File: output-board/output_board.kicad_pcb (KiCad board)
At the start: 2 copper layers, 35 parts, among them J1 Conn_Input, J2 3V3, J3 5V, J4 Channel 1-2, J5 Channel 5-6, J6 Channel 3-4, J7 Channel 7-8, U1 PCM1681

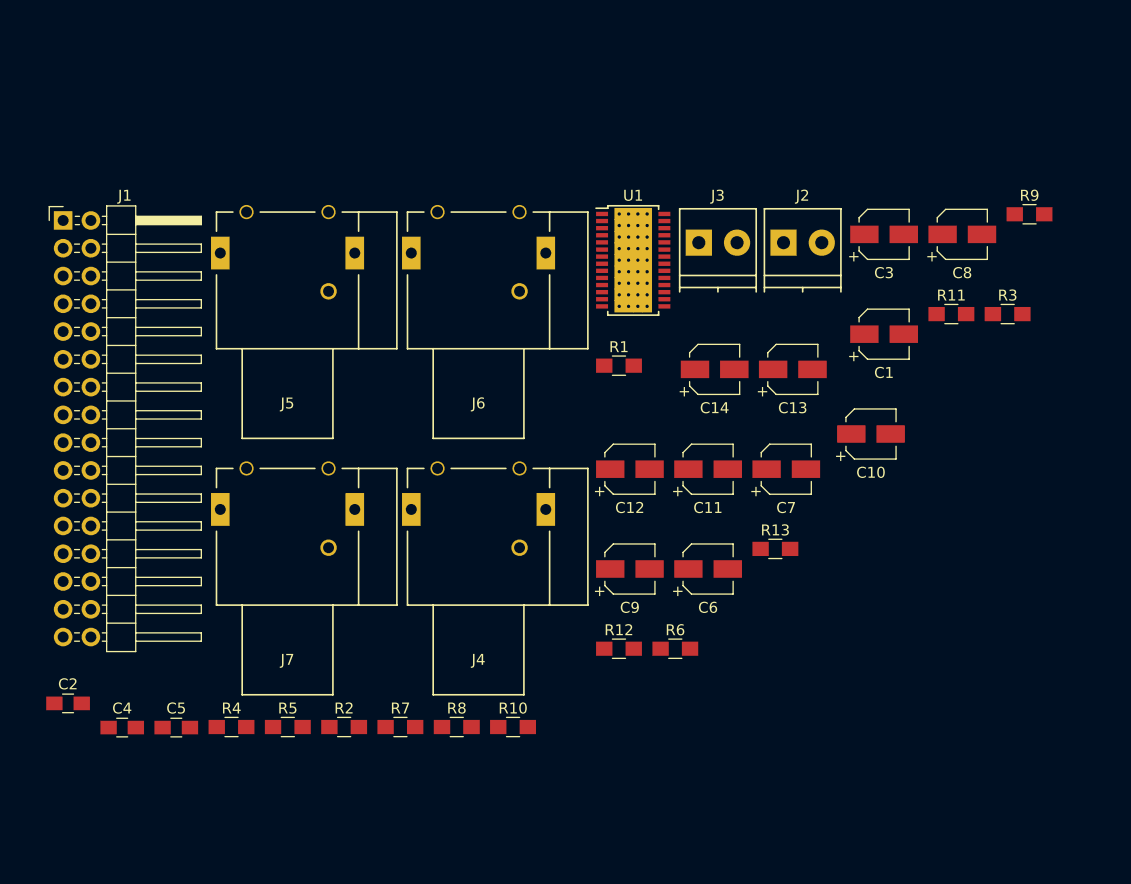
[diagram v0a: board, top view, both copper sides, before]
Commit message: update output-board
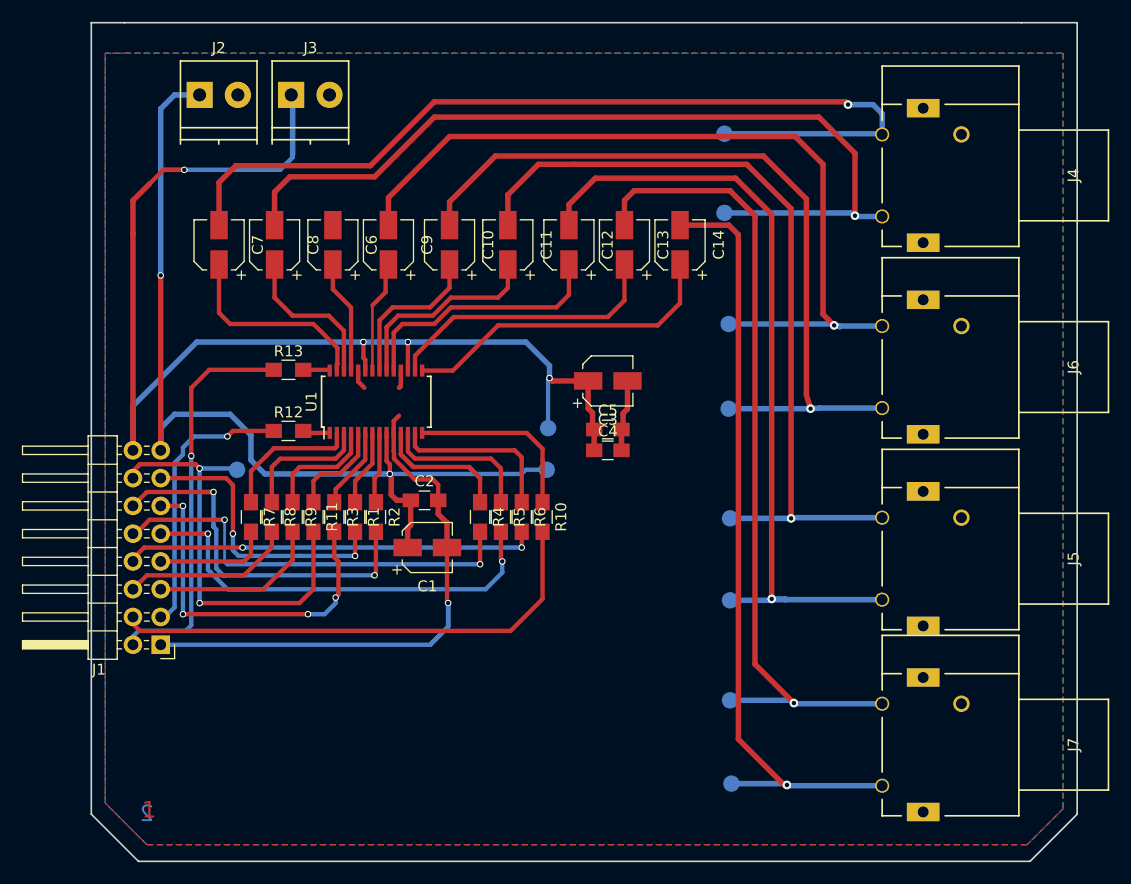
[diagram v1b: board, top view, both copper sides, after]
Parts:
- added TP1: Test_Point, Measurement_Points:Measurement_Point_Round-SMD-Pad_Small, B.Cu at (127.6, 91.9)
- added TP10: Test_Point, Measurement_Points:Measurement_Point_Round-SMD-Pad_Small, B.Cu at (172.7, 103.9)
- added TP11: Test_Point, Measurement_Points:Measurement_Point_Round-SMD-Pad_Small, B.Cu at (172.8, 120.7)
- added TP2: Test_Point, Measurement_Points:Measurement_Point_Round-SMD-Pad_Small, B.Cu at (156.0, 91.9)
- added TP3: Test_Point, Measurement_Points:Measurement_Point_Round-SMD-Pad_Small, B.Cu at (156.1, 88.1)
- added TP4: Test_Point, Measurement_Points:Measurement_Point_Round-SMD-Pad_Small, B.Cu at (172.2, 61.2)
- added TP5: Test_Point, Measurement_Points:Measurement_Point_Round-SMD-Pad_Small, B.Cu at (172.6, 78.6)
- added TP6: Test_Point, Measurement_Points:Measurement_Point_Round-SMD-Pad_Small, B.Cu at (172.2, 68.5)
- added TP7: Test_Point, Measurement_Points:Measurement_Point_Round-SMD-Pad_Small, B.Cu at (172.6, 86.4)
- added TP8: Test_Point, Measurement_Points:Measurement_Point_Round-SMD-Pad_Small, B.Cu at (172.7, 96.4)
- added TP9: Test_Point, Measurement_Points:Measurement_Point_Round-SMD-Pad_Small, B.Cu at (172.7, 113.0)
- J1: footprint Pin_Headers:Pin_Header_Angled_2x16_Pitch2.54mm -> Pin_Headers:Pin_Header_Angled_2x08_Pitch2.54mm
- moved R9 72.9 mm to (132.7, 96.3), turned to 270 degrees
- moved J5 69.6 mm to (199.1, 100.1), turned to 90 degrees
- moved J7 68.1 mm to (199.1, 117.1), turned to 90 degrees
- moved R3 64.3 mm to (136.5, 96.3), turned to 270 degrees
- moved J4 63.1 mm to (199.1, 65.0), turned to 90 degrees
- moved C8 62.9 mm to (131.1, 71.4), turned to 90 degrees
- moved R11 61.2 mm to (134.6, 96.3), turned to 270 degrees
- moved C7 55.8 mm to (126.0, 71.4), turned to 90 degrees
- moved J2 55.1 mm to (124.2, 57.7)
- moved C4 51.1 mm to (161.5, 90.2)
- moved J6 49.4 mm to (199.1, 82.5), turned to 90 degrees
- moved C5 48.0 mm to (161.5, 88.3)
- moved R13 47.4 mm to (132.3, 82.8)
- moved C1 46.1 mm to (145.0, 99.1)
- moved C6 45.4 mm to (136.4, 71.4), turned to 90 degrees
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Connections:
- C10 pad 1: /VOUT4 -> Net-(C10-Pad1)
- C10 pad 2: Net-(C10-Pad2) -> /VOUT4
- C11 pad 1: /VOUT5 -> Net-(C11-Pad1)
- C11 pad 2: Net-(C11-Pad2) -> /VOUT5
- C12 pad 1: /VOUT6 -> Net-(C12-Pad1)
- C12 pad 2: Net-(C12-Pad2) -> /VOUT6
- C13 pad 1: /VOUT7 -> Net-(C13-Pad1)
- C13 pad 2: Net-(C13-Pad2) -> /VOUT7
- C14 pad 1: /VOUT8 -> Net-(C14-Pad1)
- C14 pad 2: Net-(C14-Pad2) -> /VOUT8
- C7 pad 1: /VOUT1 -> Net-(C7-Pad1)
- C7 pad 2: Net-(C7-Pad2) -> /VOUT1
- C8 pad 1: /VOUT2 -> Net-(C8-Pad1)
- C8 pad 2: Net-(C8-Pad2) -> /VOUT2
- C9 pad 1: /VOUT3 -> Net-(C9-Pad1)
- C9 pad 2: Net-(C9-Pad2) -> /VOUT3
- U1 pad 15: Net-(C14-Pad2) -> Net-(C14-Pad1)
- U1 pad 16: Net-(C13-Pad2) -> Net-(C13-Pad1)
- U1 pad 19: Net-(C12-Pad2) -> Net-(C12-Pad1)
- U1 pad 20: Net-(C11-Pad2) -> Net-(C11-Pad1)
- U1 pad 21: Net-(C10-Pad2) -> Net-(C10-Pad1)
- U1 pad 22: Net-(C9-Pad2) -> Net-(C9-Pad1)
- U1 pad 26: Net-(C8-Pad2) -> Net-(C8-Pad1)
- U1 pad 27: Net-(C7-Pad2) -> Net-(C7-Pad1)
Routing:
- net +5VA: track 0.00 -> 113.5 mm, vias 0 -> 4
- net +3V3: track 0.00 -> 89.2 mm, vias 0 -> 2
- net /VOUT1: track 0.00 -> 84.5 mm, vias 0 -> 1
- net /VOUT2: track 0.00 -> 80.6 mm, vias 0 -> 1
- net /VOUT7: track 0.00 -> 76.3 mm, vias 0 -> 1
- net /VOUT3: track 0.00 -> 75.5 mm, vias 0 -> 1
- net /VOUT5: track 0.00 -> 73.8 mm, vias 0 -> 1
- net /VOUT6: track 0.00 -> 73.6 mm, vias 0 -> 1
- net /VOUT8: track 0.00 -> 72.1 mm, vias 0 -> 1
- net /VOUT4: track 0.00 -> 71.4 mm, vias 0 -> 1
- net GNDA: track 0.00 -> 64.3 mm, vias 0 -> 1
- net /MSEL: track 0.00 -> 46.0 mm
- net /DATA3: track 0.00 -> 39.7 mm, vias 0 -> 2
- net /DATA2: track 0.00 -> 39.2 mm, vias 0 -> 2
- net /SCK: track 0.00 -> 39.1 mm, vias 0 -> 2
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- added copper zone on B.Cu, net GNDA
- added copper zone on F.Cu, net GNDA
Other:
- board outline added: 90.2 x 76.7 mm
- net class Default: trace_width 0.25 -> 0.4
- net class alim added: clearance 0.2, trace_width 0.4, via_dia 0.6, via_drill 0.4
- net class audio_output added: clearance 0.2, trace_width 0.5, via_dia 0.8, via_drill 0.4
- board text added: "1"
- board text added: "2"
